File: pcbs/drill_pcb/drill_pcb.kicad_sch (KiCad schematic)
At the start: 25 parts, among them J1 24V IN, J10 WEIGHT SENSOR, J11 STEPPER STORAGE, J2 DC MOTOR 24 V, J3 DC MOTOR UART, J4 ENCODER VERTICAL DRIVE, J5 LIMIT SENSOR TOP, J6 HEIGHT SENSOR, J7 STEPPER VERTICAL DRIVE, J8 ENCODER STORAGE, J9 LIMIT SENSOR BOTTOM, U1 ESP32-DevKitC, U2 LM3940

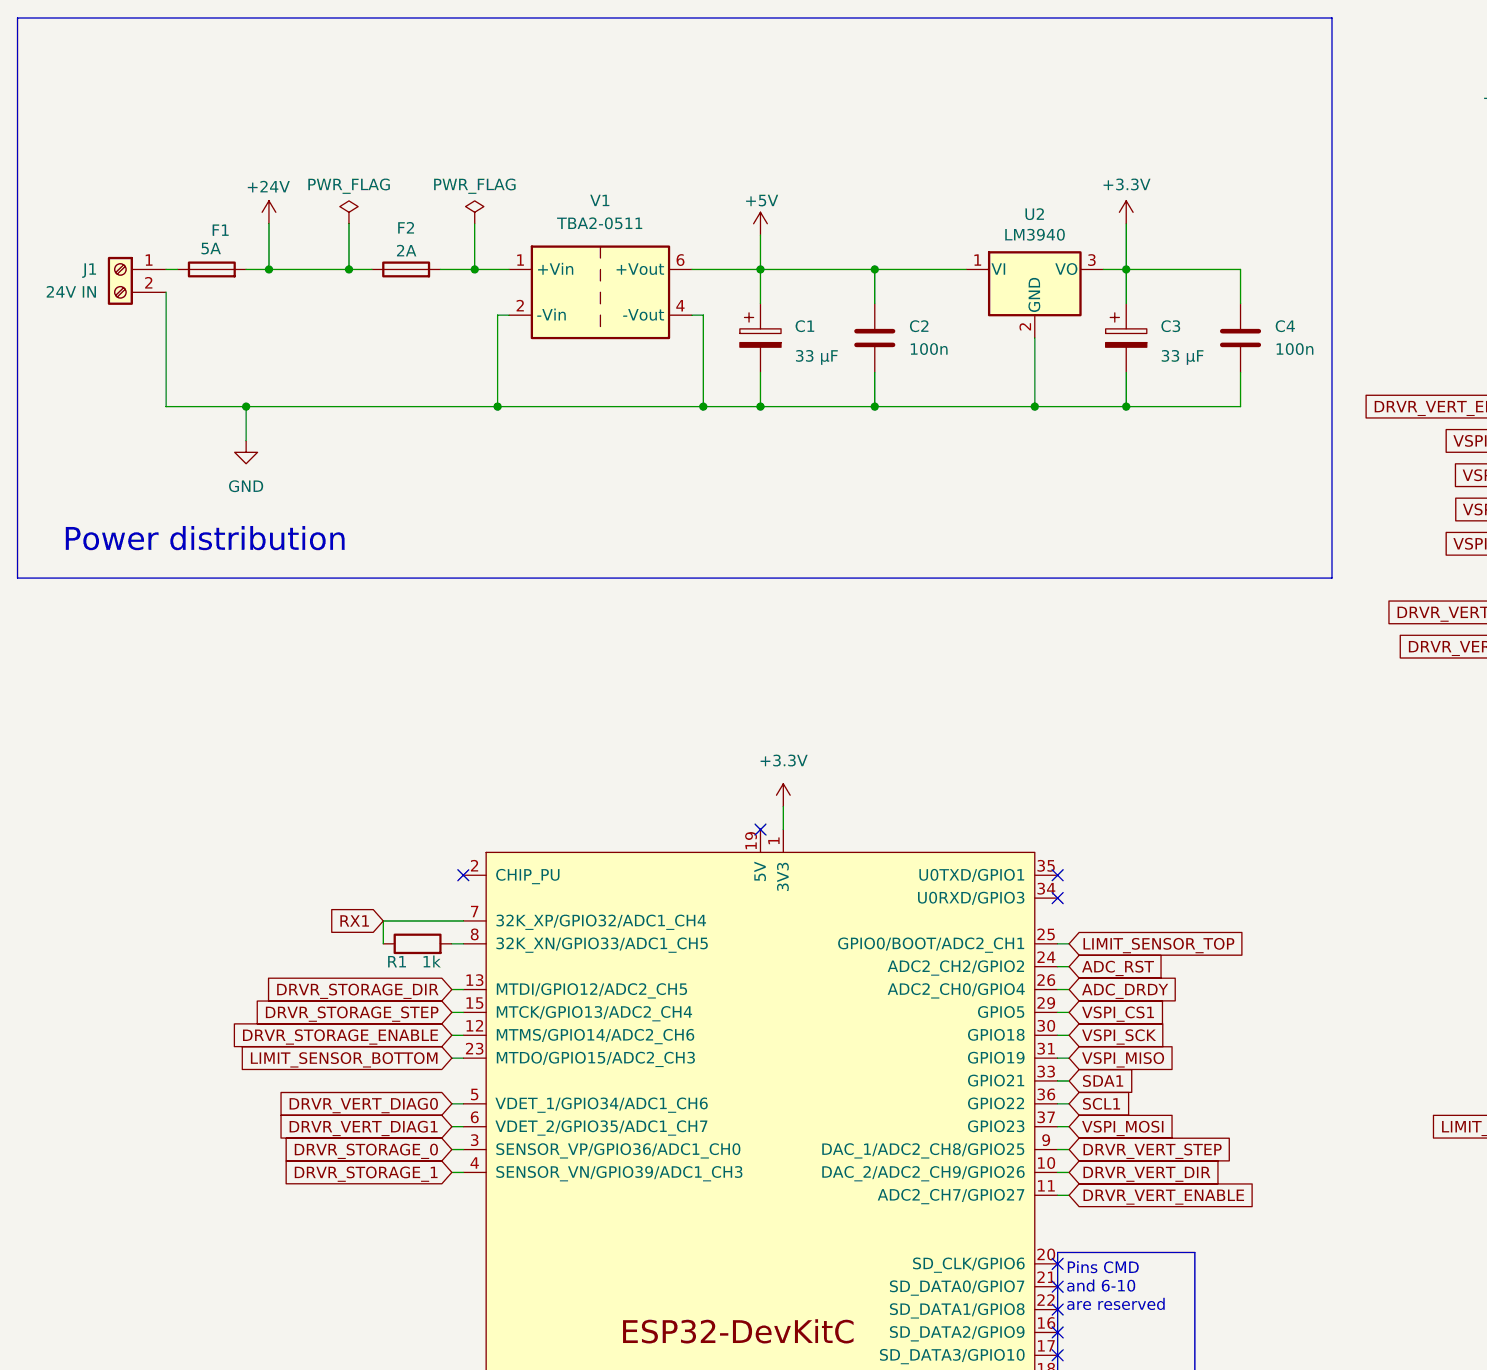
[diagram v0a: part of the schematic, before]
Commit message: PCB should be fully complete now. Somebody pls review it :(
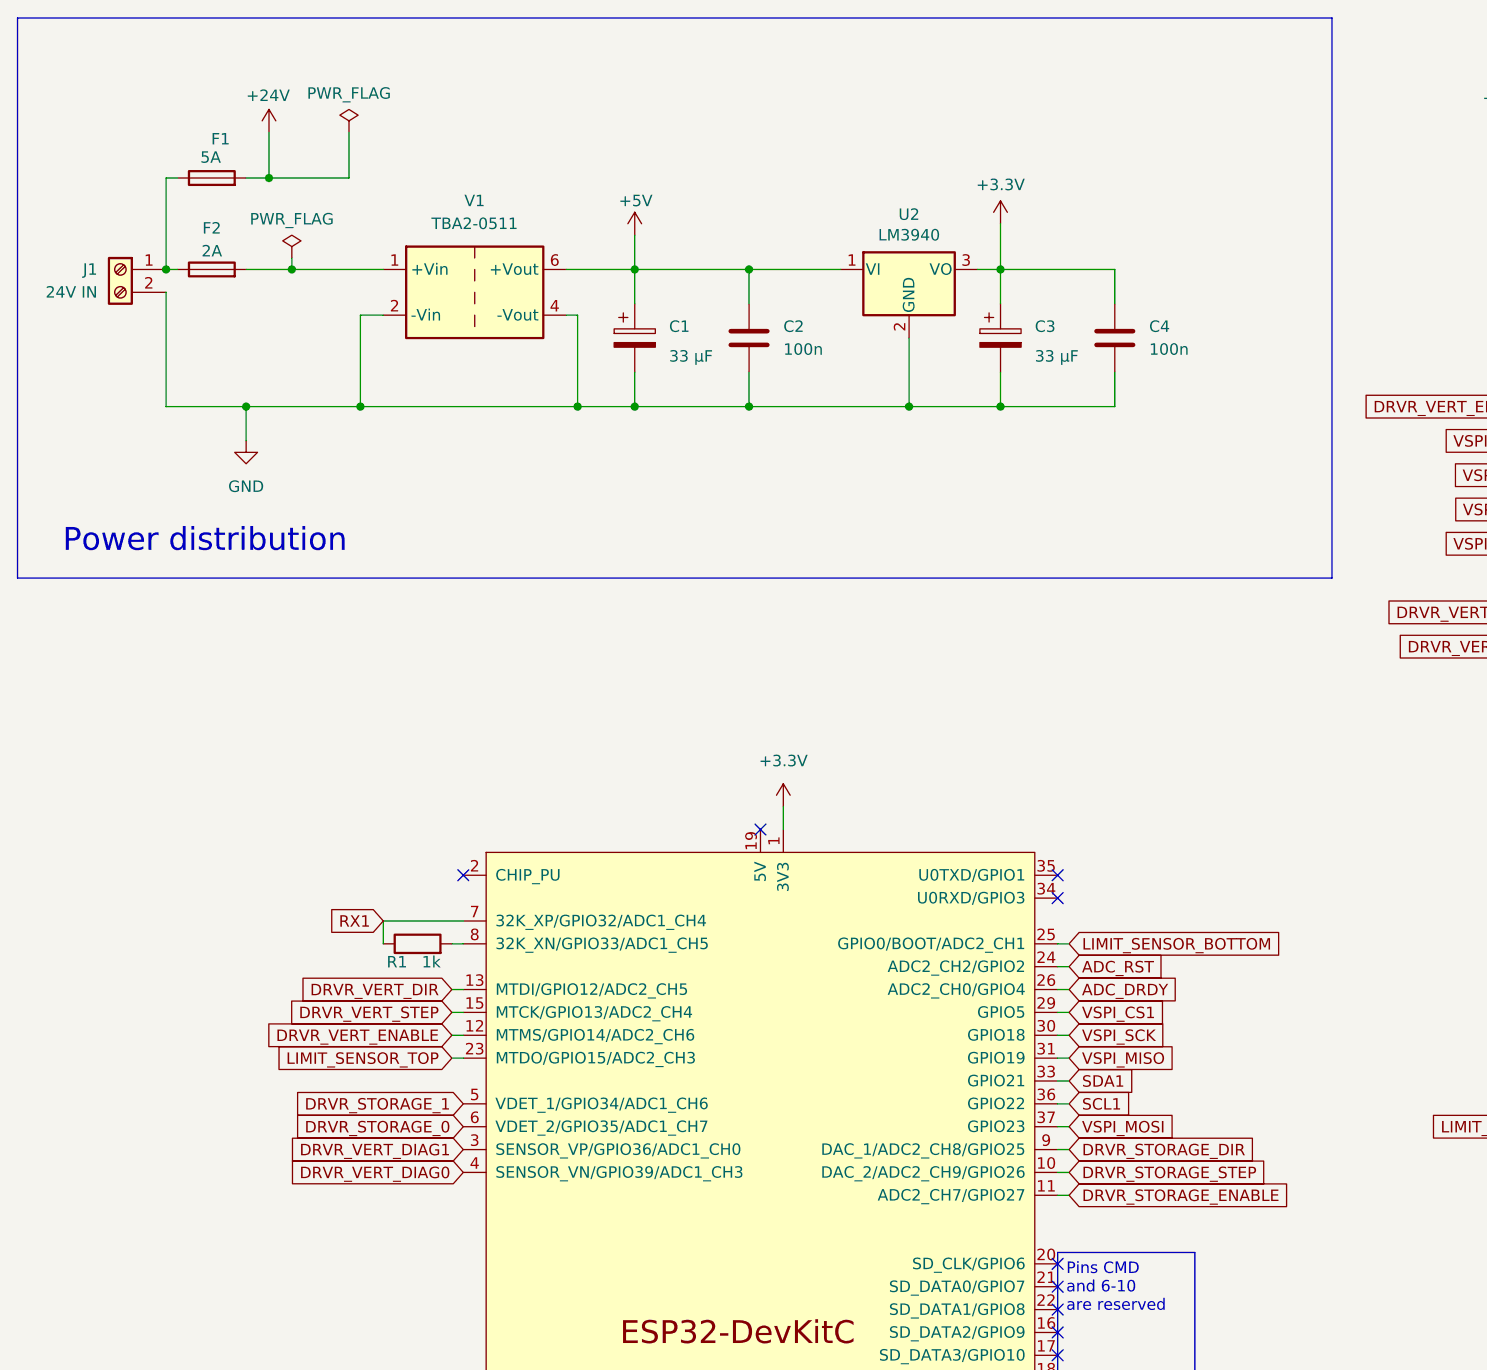
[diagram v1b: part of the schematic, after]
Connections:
- net +24V: no longer F2.1
- net DRVR_STORAGE_0: now also U1.6 (VDET_2/GPIO35/ADC1_CH7); no longer U1.3 (SENSOR_VP/GPIO36/ADC1_CH0)
- net DRVR_STORAGE_1: now also U1.5 (VDET_1/GPIO34/ADC1_CH6); no longer U1.4 (SENSOR_VN/GPIO39/ADC1_CH3)
- net DRVR_STORAGE_DIR: now also U1.9 (DAC_1/ADC2_CH8/GPIO25); no longer U1.13 (MTDI/GPIO12/ADC2_CH5)
- net DRVR_STORAGE_ENABLE: now also U1.11 (ADC2_CH7/GPIO27); no longer U1.12 (MTMS/GPIO14/ADC2_CH6)
- net DRVR_STORAGE_STEP: now also U1.10 (DAC_2/ADC2_CH9/GPIO26); no longer U1.15 (MTCK/GPIO13/ADC2_CH4)
- net DRVR_VERT_DIAG0: now also U1.4 (SENSOR_VN/GPIO39/ADC1_CH3); no longer U1.5 (VDET_1/GPIO34/ADC1_CH6)
- net DRVR_VERT_DIAG1: now also U1.3 (SENSOR_VP/GPIO36/ADC1_CH0); no longer U1.6 (VDET_2/GPIO35/ADC1_CH7)
- net DRVR_VERT_DIR: now also U1.13 (MTDI/GPIO12/ADC2_CH5); no longer U1.10 (DAC_2/ADC2_CH9/GPIO26)
- net DRVR_VERT_ENABLE: now also U1.12 (MTMS/GPIO14/ADC2_CH6); no longer U1.11 (ADC2_CH7/GPIO27)
- net DRVR_VERT_STEP: now also U1.15 (MTCK/GPIO13/ADC2_CH4); no longer U1.9 (DAC_1/ADC2_CH8/GPIO25)
- net LIMIT_SENSOR_BOTTOM: now also U1.25 (GPIO0/BOOT/ADC2_CH1); no longer U1.23 (MTDO/GPIO15/ADC2_CH3)
- net LIMIT_SENSOR_TOP: now also U1.23 (MTDO/GPIO15/ADC2_CH3); no longer U1.25 (GPIO0/BOOT/ADC2_CH1)
- net at F1.1, J1.1 (Pin_1): now also F2.1
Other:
- moved on the sheet: C1, C2, C3, C4, F1, F2, U2, V1
